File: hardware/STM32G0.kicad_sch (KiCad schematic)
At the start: 15 parts, among them T1 TP_+3V3, U1 STM32G0C1KCTxN

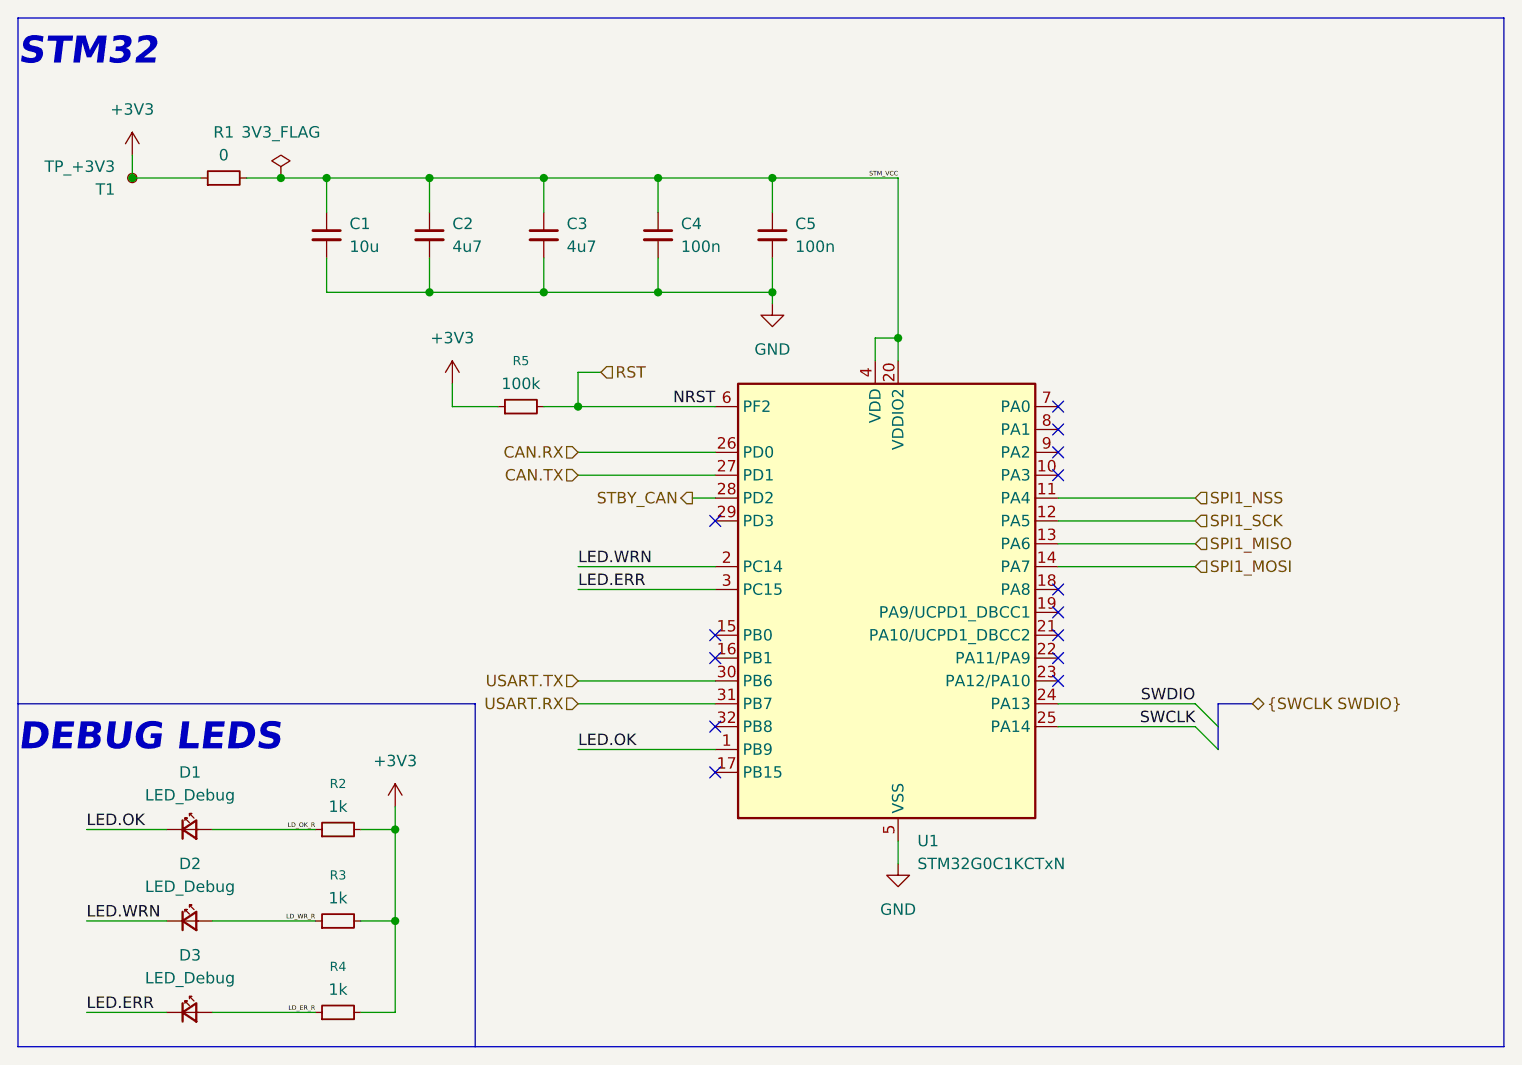
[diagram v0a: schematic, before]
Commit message: reorganization of project folders acording to templates
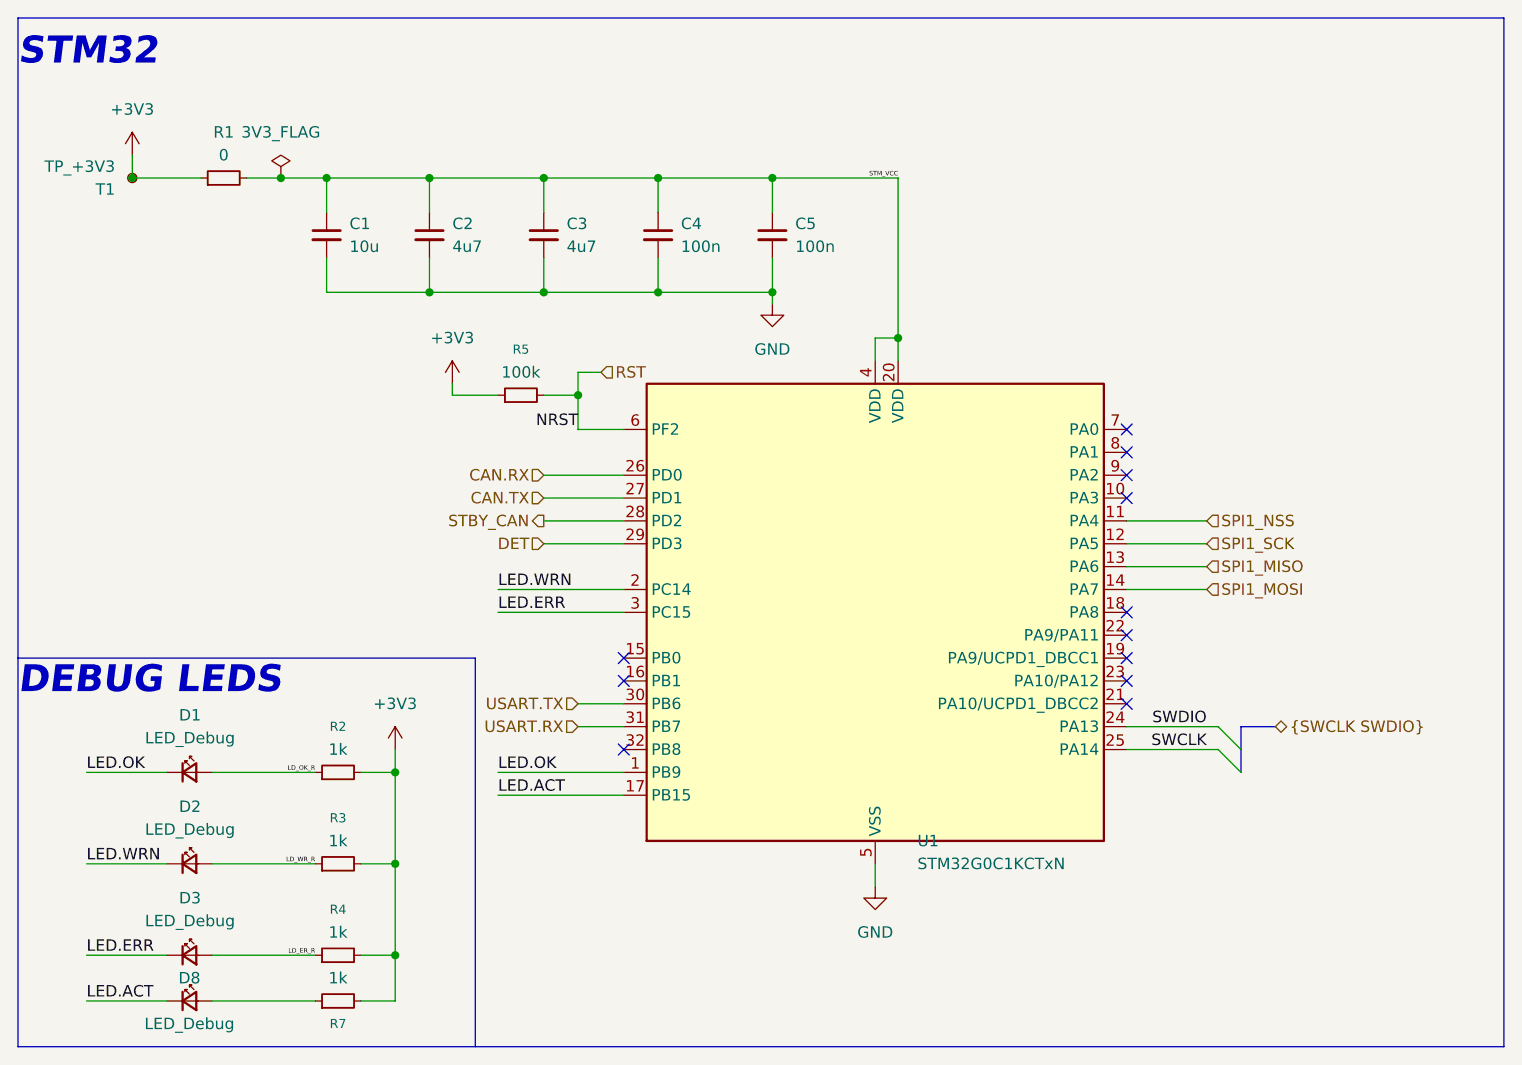
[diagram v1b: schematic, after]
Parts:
- added D8: LED_Debug, LED_SMD:LED_01005_0402Metric_Pad0.57x0.30mm_HandSolder, symbol Device:LED_Small
- added R7: 1k, Resistor_SMD:R_0603_1608Metric_Pad0.98x0.95mm_HandSolder, symbol Device:R_Small
- D1, D2, D3: footprint (none) -> LED_SMD:LED_01005_0402Metric_Pad0.57x0.30mm_HandSolder
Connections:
- net +3V3: now also R7.2
- net LED.ACT: now reaches U1.17 (PB15)
- net LED.ACT: now also D8.1 (K)
- net DET: now reaches U1.29 (PD3)
- new net: D8.2 (A), R7.1
- no-connect marks 14 -> 12
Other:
- moved on the sheet: D1, D2, D3, R2, R3, R4, R5, U1
